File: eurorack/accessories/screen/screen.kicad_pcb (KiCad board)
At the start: 2 copper layers, 10.2 x 20.6 mm, 13 parts, among them J1 Conn_01x04

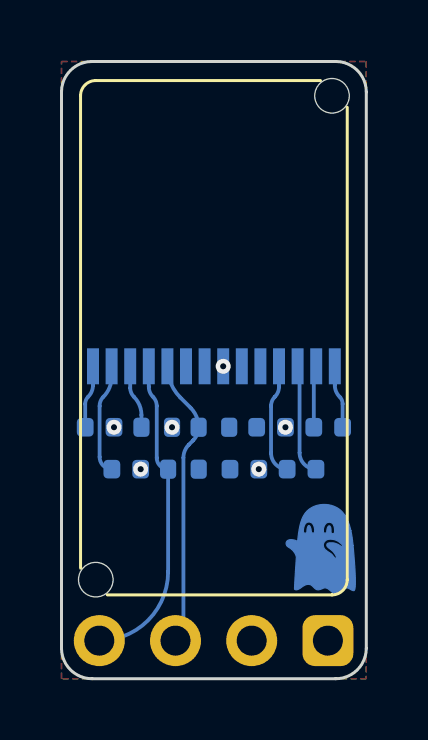
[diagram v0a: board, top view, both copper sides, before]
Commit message: jan 24
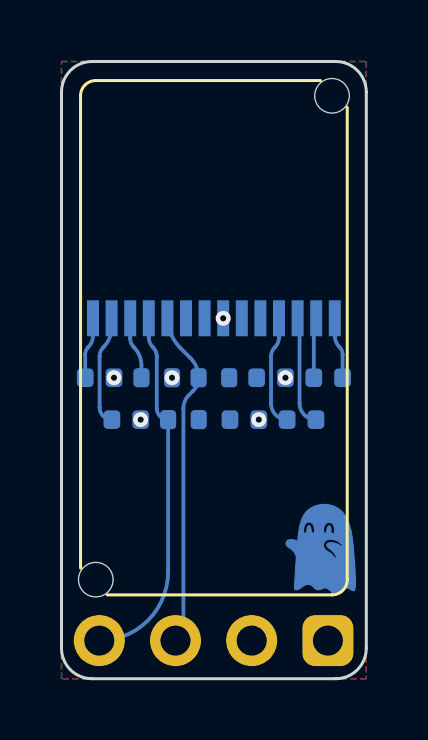
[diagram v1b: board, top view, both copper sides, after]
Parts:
- R1: value 310r -> 310K
- moved C1 1.65 mm to (135.3, 53.7)
- moved C4 1.65 mm to (127.6, 53.7)
- moved C6 1.65 mm to (133.3, 53.7)
- moved R1 1.65 mm to (129.5, 53.7)
- moved R2 1.65 mm to (131.4, 53.7)
- moved C2 1.65 mm to (134.4, 55.1)
- moved C3 1.65 mm to (132.5, 55.1)
- moved C5 1.65 mm to (128.5, 55.1)
- moved R3 1.65 mm to (130.4, 55.1)
- moved U1 1.60 mm to (131.4, 51.7)
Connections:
- U1 pad 9: unconnected-(U1-~{RES}-Pad9) -> +3.3V
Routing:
- net SDA: track 10.6 -> 12.3 mm
- net SCL: track 9.75 -> 11.4 mm
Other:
- board text added: "jan 24"
- board text removed: "oct 23"
